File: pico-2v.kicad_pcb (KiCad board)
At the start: 4 copper layers, 51.5 x 21 mm, 53 parts, among them J1 USB_C_Receptacle_USB2.0_16P, J2 VOLTSEL, J3 Header-1, J4 Header-2, J5 Conn_01x04, J6 Conn_01x04, J7 Conn_02x05_Odd_Even, SW1 UK-B0273-SP25Y, SW2 USB Boot, U1 RP2354A, U2 MCP1703T-3302E/CB, U3 MCP1703T-1802E/CB, U4 TLV71311PDBVR, U5 LMV331, Y1 ECS-3225MV-120-BN-TR3

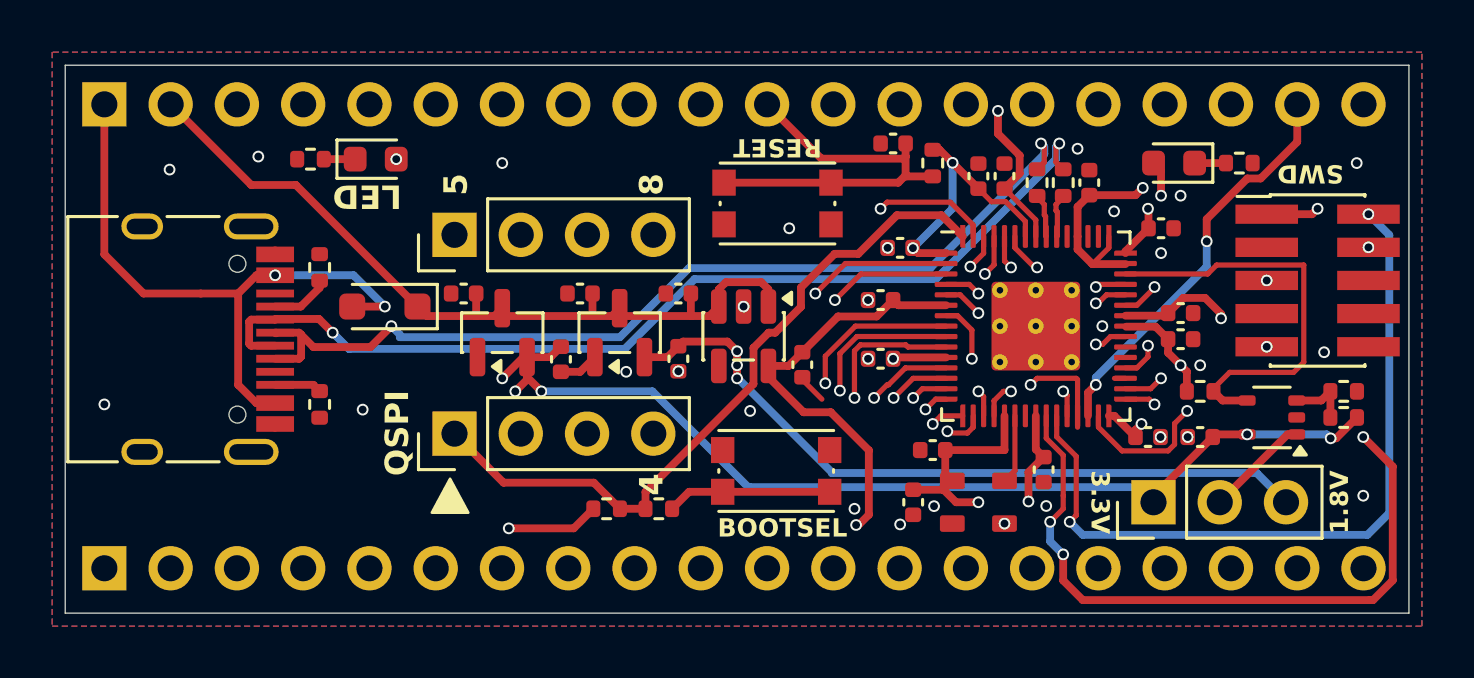
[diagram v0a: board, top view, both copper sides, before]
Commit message: Bug fixes
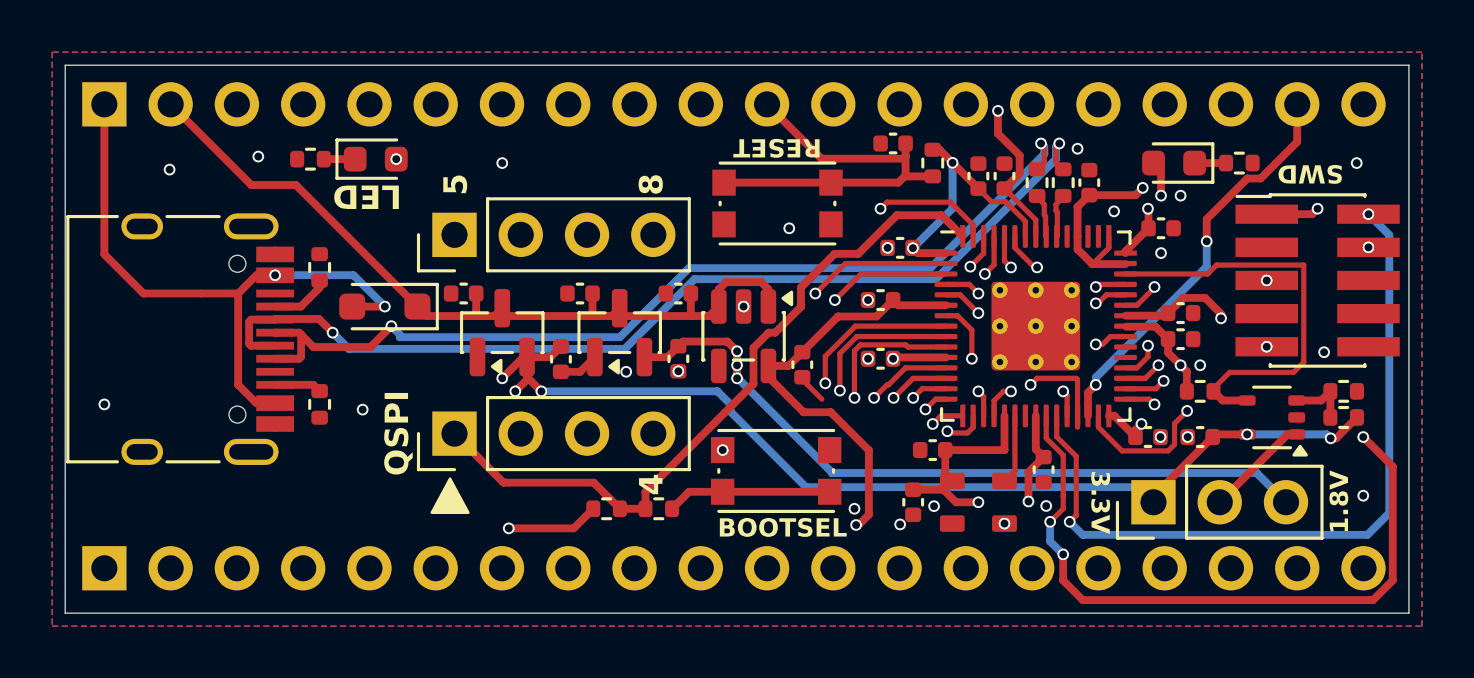
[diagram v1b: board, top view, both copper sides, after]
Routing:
- net GPIO21: track 18.8 -> 17.2 mm
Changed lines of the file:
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@@
 	)
 	(segment
-		(start 164.629904 104.669904)
-		(end 165.21 105.25)
+		(start 141.75 101)
+		(end 148.5 101)
 		(width 0.3)
 		(layer "B.Cu")
@@
 	)
 	(segment
-		(start 149.73343 104.669904)
+		(start 151.890672 104.669904)
 		(end 164.629904 104.669904)
 		(width 0.3)
@@
 	)
 	(segment
-		(start 172 102.8)
-		(end 171.85 102.65)
+		(start 164.629904 104.669904)
+		(end 165.21 105.25)
 		(width 0.3)
 		(layer "B.Cu")
@@
 	)
 	(segment
-		(start 171.85 102.65)
-		(end 168.8 102.65)
+		(start 149 101.779232)
+		(end 151.890672 104.669904)
+		(width 0.3)
+		(layer "B.Cu")
+		(net 1)
+	)
+	(segment
+		(start 172 102.8)
+		(end 171.85 102.65)
 		(width 0.3)
 		(layer "B.Cu")
@@
 	)
 	(segment
-		(start 149.704334 104.699)
-		(end 146.005334 101)
+		(start 171.85 102.65)
+		(end 168.8 102.65)
 		(width 0.3)
 		(layer "B.Cu")
@@
 	)
 	(segment
-		(start 146.005334 101)
-		(end 141.75 101)
+		(start 148.5 101)
+		(end 149 101.5)
 		(width 0.3)
 		(layer "B.Cu")
@@
 	)
 	(segment
-		(start 149.704334 104.699)
-		(end 149.73343 104.669904)
+		(start 149 101.5)
+		(end 149 101.779232)
 		(width 0.3)
 		(layer "B.Cu")
@@
 	)
 	(via
-		(at 149.75 101.75)
-		(size 0.45)
-		(drill 0.3)
-		(layers "F.Cu" "B.Cu")
-		(free yes)
-		(net 2)
-	)
-	(via
 		(at 166.25 93.5)
 		(size 0.45)
@@
 	)
 	(via
+		(at 148.7 103.25)
+		(size 0.45)
+		(drill 0.3)
+		(layers "F.Cu" "B.Cu")
+		(net 2)
+	)
+	(via
 		(at 155.02 95.5)
 		(size 0.45)
@@
 	)
 	(segment
+		(start 149.25 99.46296)
+		(end 149.25 100.5)
+		(width 0.3)
+		(layer "B.Cu")
+		(net 6)
+	)
+	(segment
 		(start 169.169 104.129)
 		(end 152.879 104.129)
@@
 	)
 	(segment
-		(start 149.25 99.46296)
-		(end 149.25 100.5)
-		(width 0.3)
-		(layer "In2.Cu")
-		(net 6)
-	)
-	(segment
 		(start 155.71 92)
 		(end 155.71 92.72)
@@
 	)
 	(segment
-		(start 149.904616 103.75)
-		(end 150.592232 103.062384)
+		(start 136.044334 103.801)
+		(end 135.993334 103.75)
 		(width 0.3)
 		(layer "In1.Cu")
@@
 	)
 	(segment
-		(start 135.993334 103.75)
-		(end 149.904616 103.75)
+		(start 149.853616 103.801)
+		(end 136.044334 103.801)
 		(width 0.3)
 		(layer "In1.Cu")
@@
 	(segment
 		(start 133.084334 106.659)
-		(end 135.993334 103.75)
+		(end 128.661 106.659)
 		(width 0.3)
 		(layer "In1.Cu")
@@
 	)
 	(segment
-		(start 150.592232 103.062384)
-		(end 150.592232 99.907768)
+		(start 128.661 106.659)
+		(end 127.54 107.78)
 		(width 0.3)
 		(layer "In1.Cu")
@@
 	)
 	(segment
-		(start 127.54 107.78)
-		(end 128.661 106.659)
+		(start 150.592232 99.907768)
+		(end 150.592232 103.062384)
 		(width 0.3)
 		(layer "In1.Cu")
@@
 	)
 	(segment
-		(start 128.661 106.659)
-		(end 133.084334 106.659)
+		(start 153 97.5)
+		(end 150.592232 99.907768)
 		(width 0.3)
 		(layer "In1.Cu")
@@
 	)
 	(segment
-		(start 150.592232 99.907768)
-		(end 153 97.5)
+		(start 150.592232 103.062384)
+		(end 149.853616 103.801)
+		(width 0.3)
+		(layer "In1.Cu")
+		(net 24)
+	)
+	(segment
+		(start 135.993334 103.75)
+		(end 133.084334 106.659)
 		(width 0.3)
 		(layer "In1.Cu")
@@
 	)
 	(segment
+		(start 164.9 100.5)
+		(end 165.4 100)
+		(width 0.2)
+		(layer "F.Cu")
+		(net 33)
+	)
+	(segment
 		(start 164.1375 100.5)
-		(end 163.715362 100.5)
+		(end 164.9 100.5)
 		(width 0.2)
 		(layer "F.Cu")
@@
 	)
 	(via
-		(at 163.25 98.5)
+		(at 165.4 100)
 		(size 0.45)
 		(drill 0.3)
@@
 	)
 	(segment
-		(start 165.699 99.801)
-		(end 165.75 99.75)
-		(width 0.3)
-		(layer "In1.Cu")
-		(net 33)
-	)
-	(segment
 		(start 166.222 95.422)
 		(end 165.4 94.6)
@@
 	)
 	(segment
-		(start 165.75 99.75)
-		(end 165.75 99.095384)
-		(width 0.3)
-		(layer "In1.Cu")
-		(net 33)
-	)
-	(segment
 		(start 165.4 94.6)
 		(end 164.820768 94.6)
@@
 	)
 	(segment
-		(start 164.551 99.801)
-		(end 165.699 99.801)
-		(width 0.3)
-		(layer "In1.Cu")
-		(net 33)
-	)
-	(segment
-		(start 163.25 98.5)
-		(end 164.551 99.801)
+		(start 165.75 99.65)
+		(end 165.4 100)
 		(width 0.3)
 		(layer "In1.Cu")
@@
 	)
 	(segment
+		(start 165.75 99.095384)
+		(end 165.75 99.65)
+		(width 0.3)
+		(layer "In1.Cu")
+		(net 33)
+	)
+	(segment
 		(start 163.1 96.9)
 		(end 163 97)
@@
 	)
 	(segment
-		(start 165.1 100.9)
-		(end 165.5 100.5)
+		(start 164.1375 100.9)
+		(end 165.3 100.9)
 		(width 0.2)
 		(layer "F.Cu")
@@
 	)
 	(segment
-		(start 164.1375 100.9)
-		(end 165.1 100.9)
+		(start 165.3 100.9)
+		(end 165.6 100.6)
 		(width 0.2)
 		(layer "F.Cu")
@@
 	)
 	(via
-		(at 165.5 100.5)
+		(at 165.6 100.6)
 		(size 0.45)
 		(drill 0.3)
@@
 		(width 0.3)
 		(layer "In1.Cu")
-		(net 37)
-	)
-	(segment
-		(start 165.6 100.6)
-		(end 165.5 100.5)
-		(width 0.3)
-		(layer "In1.Cu")
